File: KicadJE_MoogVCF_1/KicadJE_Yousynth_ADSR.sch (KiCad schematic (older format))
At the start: 52 parts, among them J301 ADSRGate, J302 ADSR, P301 Doepfer_Power_10pin, Q301 SI2302, Q302 MMBT3904, Q303 MMBT3904, Q304 MMBT3904, SW301 SW_DPDT_x2, SW302 Gate, U301 TL072, U302 TLC555

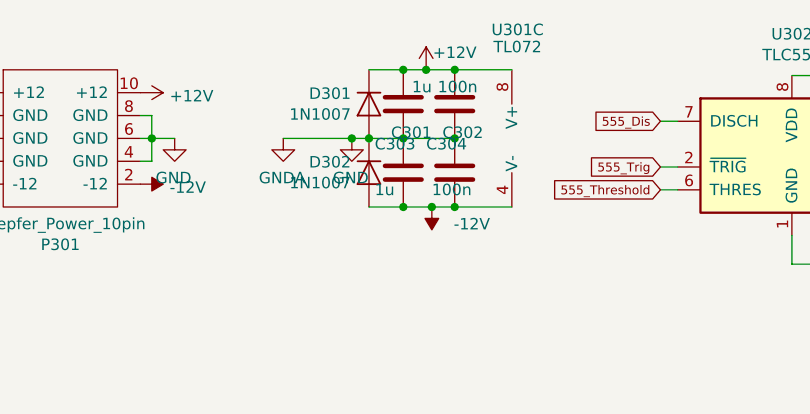
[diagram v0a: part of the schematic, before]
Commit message: ERC done
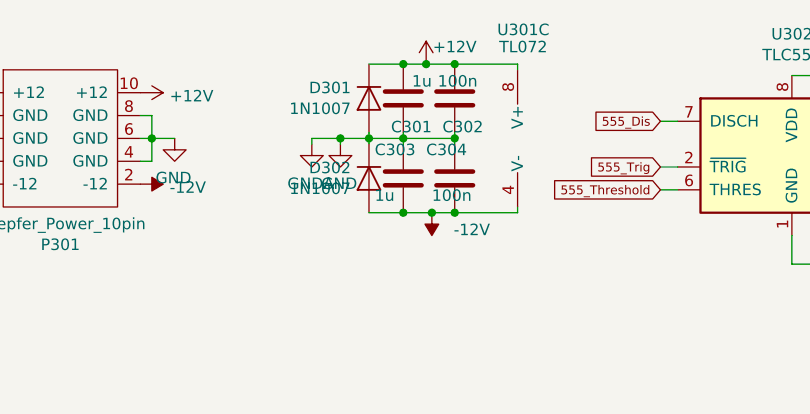
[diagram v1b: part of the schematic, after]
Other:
- moved on the sheet: C301, C302, C303, C304, D301, D302, U301C
